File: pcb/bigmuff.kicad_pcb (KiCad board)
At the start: 2 copper layers, 107.9 x 81.3 mm, 46 parts, among them Q1 BC549, Q2 BC549, Q3 BC549, Q4 BC549

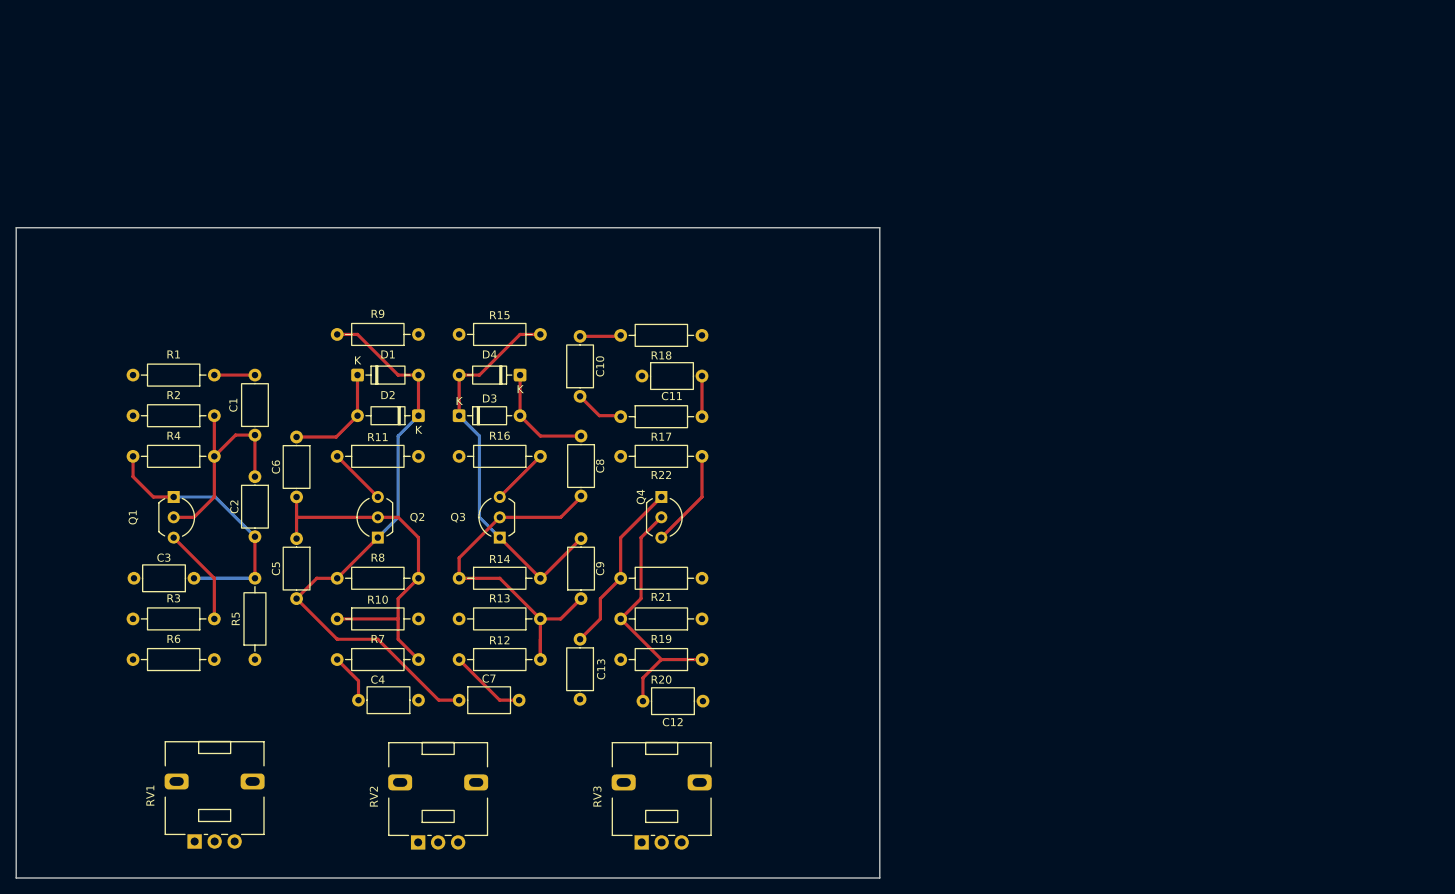
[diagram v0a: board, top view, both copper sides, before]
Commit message: updated pcb
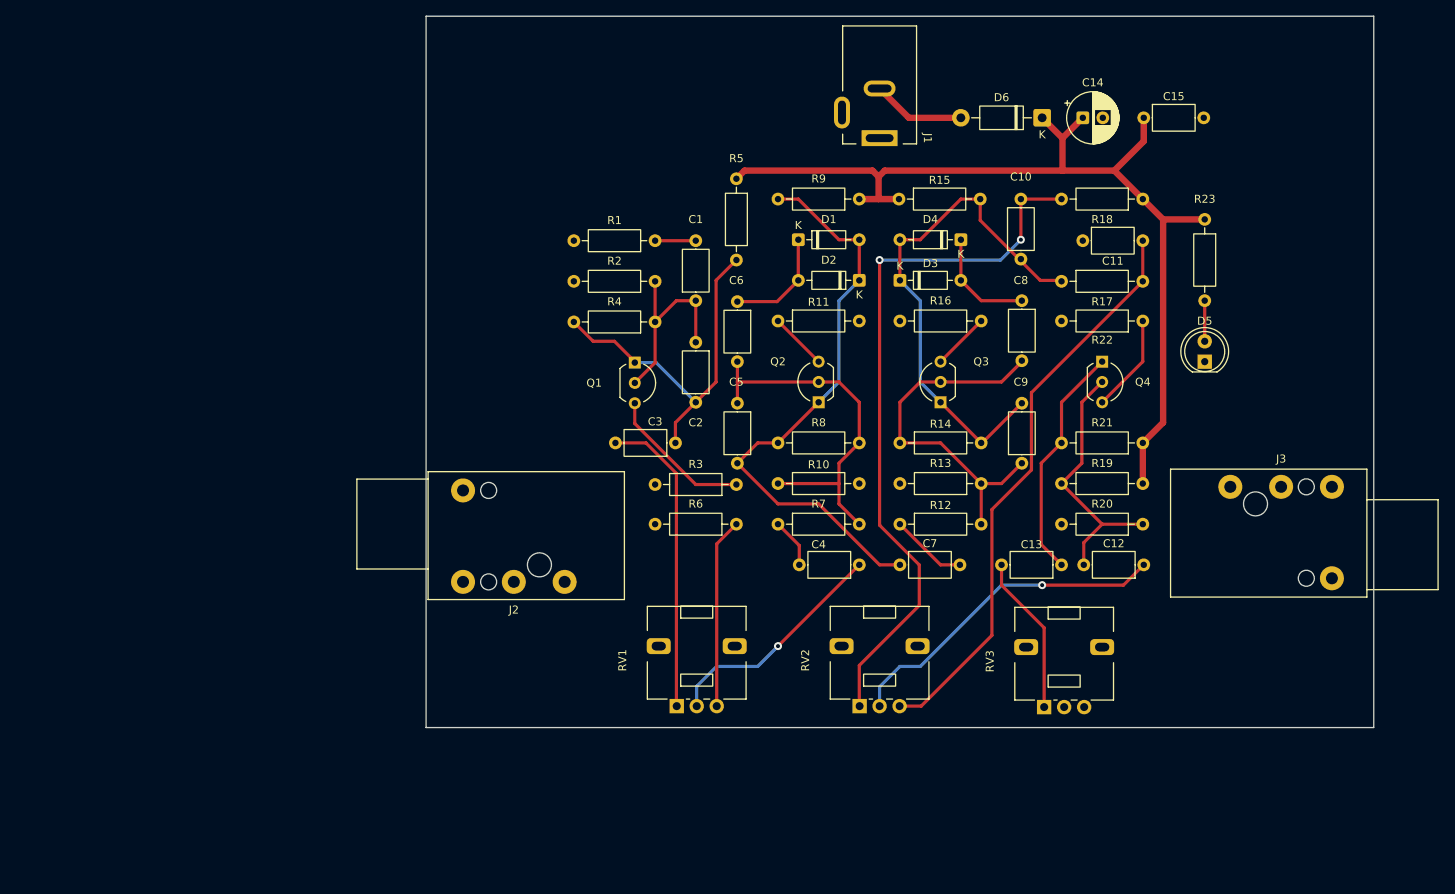
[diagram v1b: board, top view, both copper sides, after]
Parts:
- added C14: 100uF, Capacitor_THT:CP_Radial_D6.3mm_P2.50mm, F.Cu at (192.4, 56.7)
- added C15: 100nF, Capacitor_THT:C_Axial_L5.1mm_D3.1mm_P7.50mm_Horizontal, F.Cu at (200.0, 56.7)
- added D5: LED, LED_THT:LED_D5.0mm, F.Cu at (207.6, 87.2)
- added D6: 1N5817, Diode_THT:D_DO-41_SOD81_P10.16mm_Horizontal, F.Cu at (187.3, 56.7)
- added J1: Jack-DC, Connector_BarrelJack:BarrelJack_Kycon_KLDX-0202-xC_Horizontal, F.Cu at (167.0, 59.3)
- added J2: AudioJack2, Connector_Audio:Jack_6.35mm_Neutrik_NRJ3HF-1_Horizontal, F.Cu at (127.6, 114.8)
- added J3: AudioJack2, Connector_Audio:Jack_6.35mm_Neutrik_NRJ3HF-1_Horizontal, F.Cu at (210.8, 102.9)
- added R23: 4.7k, Resistor_THT:R_Axial_DIN0207_L6.3mm_D2.5mm_P10.16mm_Horizontal, F.Cu at (207.6, 69.4)
- moved R5 85.1 mm to (149.1, 64.4), turned to -90 degrees
- moved R6 67.4 mm to (149.1, 107.5)
- moved R3 67.4 mm to (149.1, 102.6)
- moved RV1 62.6 mm to (141.6, 130.3)
- moved C3 62.5 mm to (141.5, 97.4)
- moved C13 60.9 mm to (189.7, 112.6), turned to 180 degrees
- moved Q1 60.0 mm to (136.4, 87.3)
- moved RV2 57.8 mm to (164.5, 130.3)
- moved C10 57.7 mm to (184.6, 74.4)
- moved C12 57.7 mm to (200.0, 112.6)
- moved R18 57.7 mm to (199.9, 66.9)
- moved Q4 57.6 mm to (194.8, 87.2)
- moved C7 57.6 mm to (169.5, 112.6)
- moved D3 57.6 mm to (169.5, 77.1)
- moved Q2 57.6 mm to (159.4, 92.3)
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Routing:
- net VDD: track 0.00 -> 123.4 mm
- net Net-(C10-Pad2): track 5.13 -> 89.8 mm, vias 0 -> 2
- net Net-(C11-Pad2): track 5.08 -> 72.4 mm
- net TONE_OUT: track 0.00 -> 41.8 mm, vias 0 -> 1
- net Net-(C3-Pad2): track 0.00 -> 38.3 mm
- net BOOST_OUT: track 0.00 -> 29.1 mm, vias 0 -> 1
- net Net-(R6-Pad1): track 0.00 -> 23.8 mm
- net Net-(C13-Pad2): track 0.00 -> 20.0 mm
- net Net-(Q1-C): track 33.7 -> 45.5 mm, vias 1 -> 0
- net Net-(D6-A): track 0.00 -> 11.7 mm
- net CLIP_OUT: track 55.1 -> 64.8 mm
- net Net-(Q4-C): track 22.0 -> 29.6 mm
- net Net-(Q1-E): track 12.3 -> 18.4 mm
- net Net-(D5-A): track 0.00 -> 5.08 mm
- net Net-(Q1-B): track 27.7 -> 25.1 mm
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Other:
- board size 107.9 x 81.3 mm -> 118.5 x 88.9 mm

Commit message: updated pcb
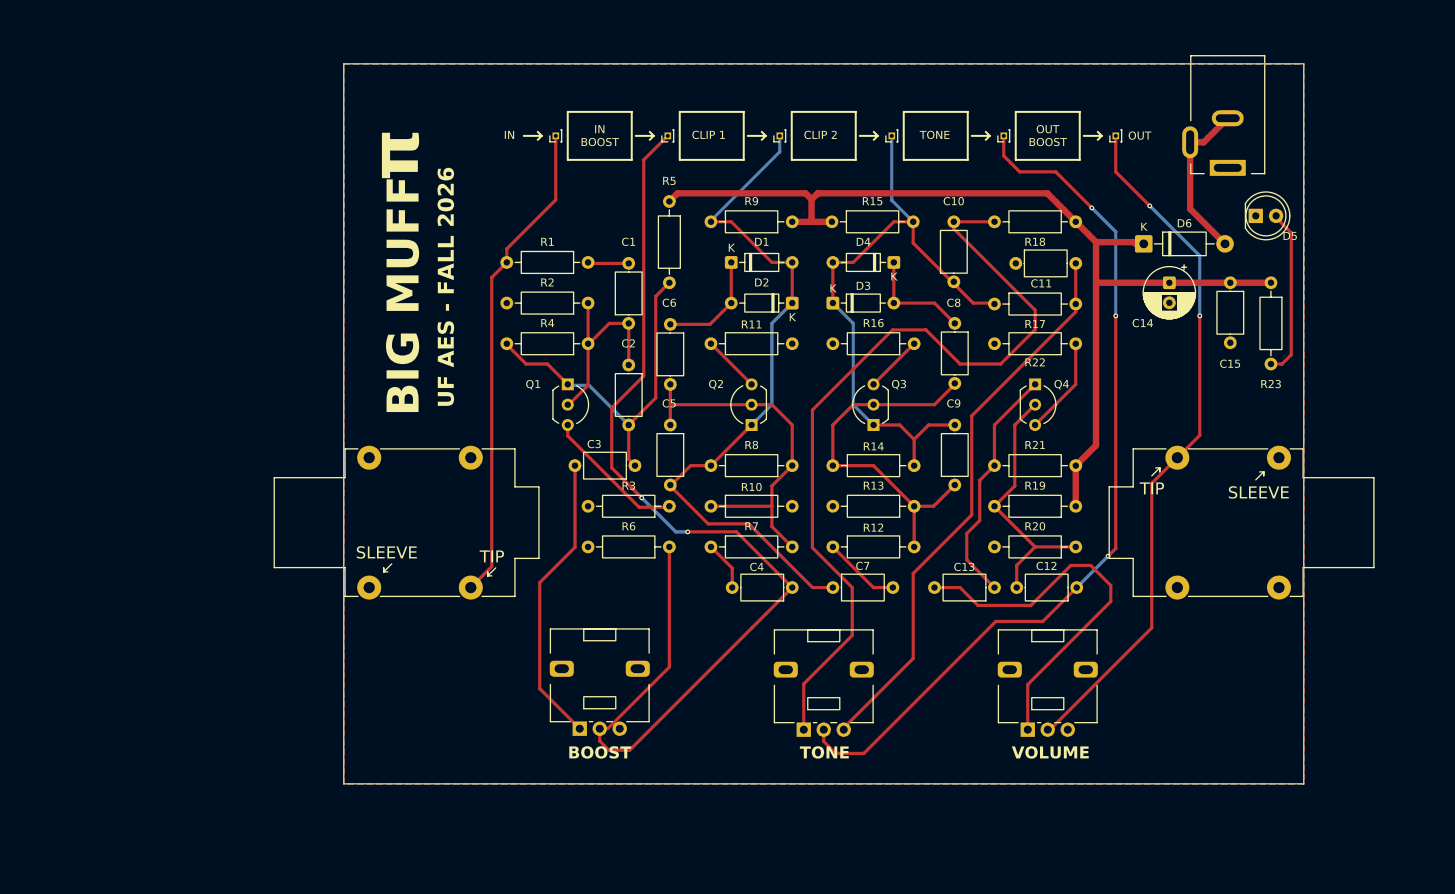
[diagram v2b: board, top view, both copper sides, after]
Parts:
- removed J3: AudioJack2, Connector_Audio:Jack_6.35mm_Neutrik_NRJ3HF-1_Horizontal
- added J4: Barrel_Jack_Switch, Connector_BarrelJack:BarrelJack_Kycon_KLDX-0202-xC_Horizontal, F.Cu at (210.5, 63.0)
- added TP1: Input, Connector_PinHeader_1.00mm:PinHeader_1x01_P1.00mm_Vertical, F.Cu at (126.5, 59.0)
- added TP2: Boost, Connector_PinHeader_1.00mm:PinHeader_1x01_P1.00mm_Vertical, F.Cu at (140.5, 59.0)
- added TP3: Clip 1, Connector_PinHeader_1.00mm:PinHeader_1x01_P1.00mm_Vertical, F.Cu at (154.5, 59.0)
- added TP4: Clip 2, Connector_PinHeader_1.00mm:PinHeader_1x01_P1.00mm_Vertical, F.Cu at (168.5, 59.0)
- added TP5: Tone, Connector_PinHeader_1.00mm:PinHeader_1x01_P1.00mm_Vertical, F.Cu at (182.5, 59.0)
- added TP6: Output, Connector_PinHeader_1.00mm:PinHeader_1x01_P1.00mm_Vertical, F.Cu at (196.5, 59.0)
- J1: value Jack-DC -> NRJ4HF; footprint Connector_BarrelJack:BarrelJack_Kycon_KLDX-0202-xC_Horizontal -> Connector_Audio:Jack_6.35mm_Neutrik_NMJ4HFD3_Horizontal
- J2: value AudioJack2 -> NRJ4HF; footprint Connector_Audio:Jack_6.35mm_Neutrik_NRJ3HF-1_Horizontal -> Connector_Audio:Jack_6.35mm_Neutrik_NMJ4HFD3_Horizontal
- moved J2 78.1 mm to (204.2, 99.2), turned to 0 degrees
- moved J1 75.9 mm to (115.9, 115.5), turned to 180 degrees
- moved C14 23.3 mm to (203.2, 77.4), turned to -90 degrees
- moved C15 23.3 mm to (210.8, 77.4), turned to -90 degrees
- moved D6 20.2 mm to (200.0, 72.5), turned to 0 degrees
- moved D5 19.3 mm to (214.0, 69.0), turned to 0 degrees
- moved RV1 12.4 mm to (129.5, 133.1)
- moved R23 11.5 mm to (215.9, 77.4)
- moved D3 8.85 mm to (161.1, 79.9)
- moved Q2 8.85 mm to (151.0, 95.1)
- moved Q4 8.85 mm to (186.4, 90.1)
- moved R14 8.85 mm to (161.1, 100.2)
- moved R5 8.85 mm to (140.7, 67.2)
- moved C7 8.85 mm to (161.1, 115.5)
- moved R12 8.85 mm to (161.1, 110.4)
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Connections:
- J2 pad S: unconnected-(J2-PadS) -> GND
- J2 pad T: unconnected-(J2-PadT) -> OUT
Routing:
- net OUT: track 0.00 -> 86.6 mm, vias 0 -> 2
- net BOOST_OUT: track 29.1 -> 107.6 mm, vias 1 -> 2
- net TONE_OUT: track 41.8 -> 109.3 mm, vias 1 -> 3
- net IN: track 0.00 -> 60.9 mm
- net Net-(C13-Pad2): track 20.0 -> 48.4 mm
- net Net-(D5-A): track 5.08 -> 21.2 mm
- net Net-(D1-A): track 73.6 -> 88.0 mm
- net Net-(C10-Pad2): track 89.8 -> 102.8 mm, vias 2 -> 0
- net CLIP_OUT: track 64.8 -> 77.3 mm
- net Net-(D6-A): track 11.7 -> 21.4 mm
- net VDD: track 123.4 -> 126.8 mm
- net Net-(R6-Pad1): track 23.8 -> 25.9 mm
- net Net-(C11-Pad2): track 72.4 -> 70.3 mm
- net Net-(C3-Pad2): track 38.3 -> 36.8 mm
- net Net-(Q4-C): track 29.6 -> 30.4 mm
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- added copper zone on B.Cu, net GND
- added copper zone on F.Cu, net GND
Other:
- board size 118.5 x 88.9 mm -> 120 x 90 mm
- board text added: "BIG MUFF"
- board text added: "BOOST"
- board text added: "CLIP 1"
- board text added: "CLIP 2"
- board text added: "IN"
- board text added: "IN BOOST"
- board text added: "OUT"
- board text added: "OUT BOOST"
- board text added: "SLEEVE"
- board text added: "TIP"
- board text added: "TONE"
- board text added: "UF AES - FALL 2026"
- board text added: "VOLUME"
- board text added: "π"
